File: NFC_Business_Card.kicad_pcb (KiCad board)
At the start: 2 copper layers, 85.6 x 54 mm, 7 parts

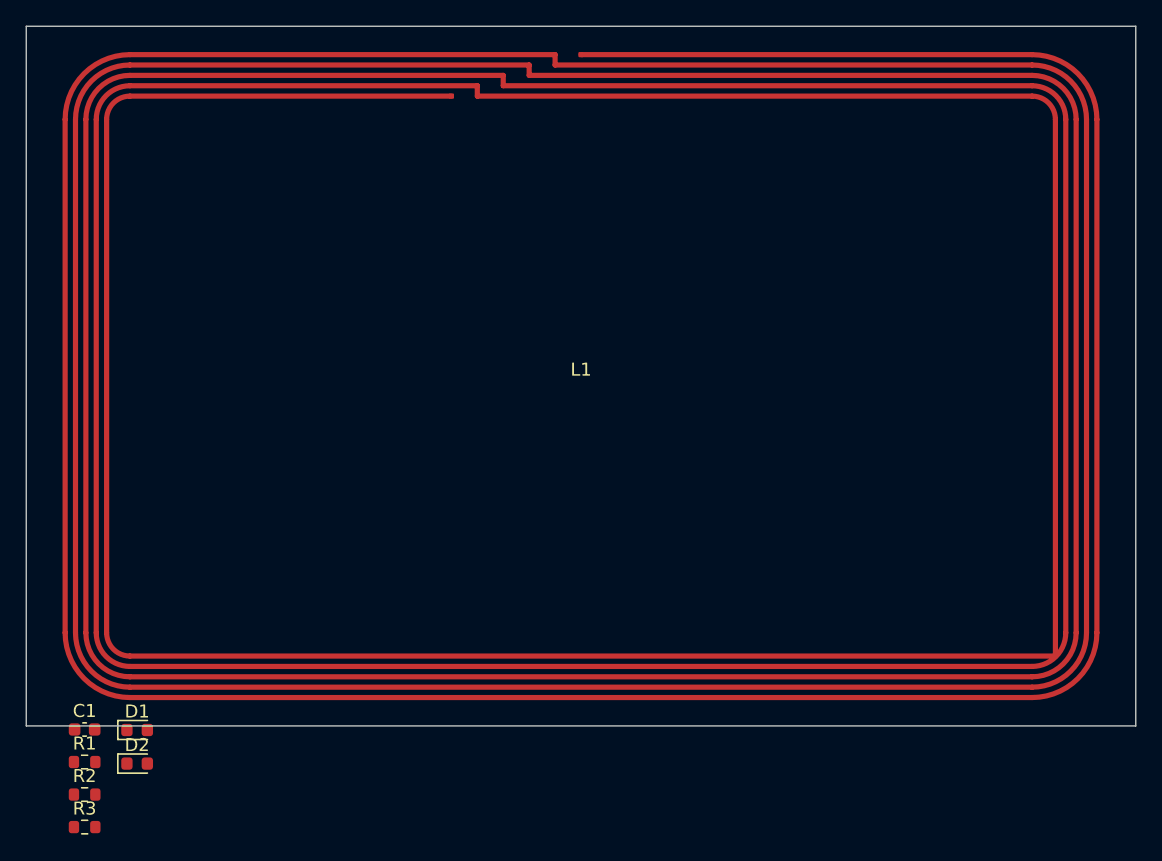
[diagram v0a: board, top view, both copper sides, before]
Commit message: Placed most components
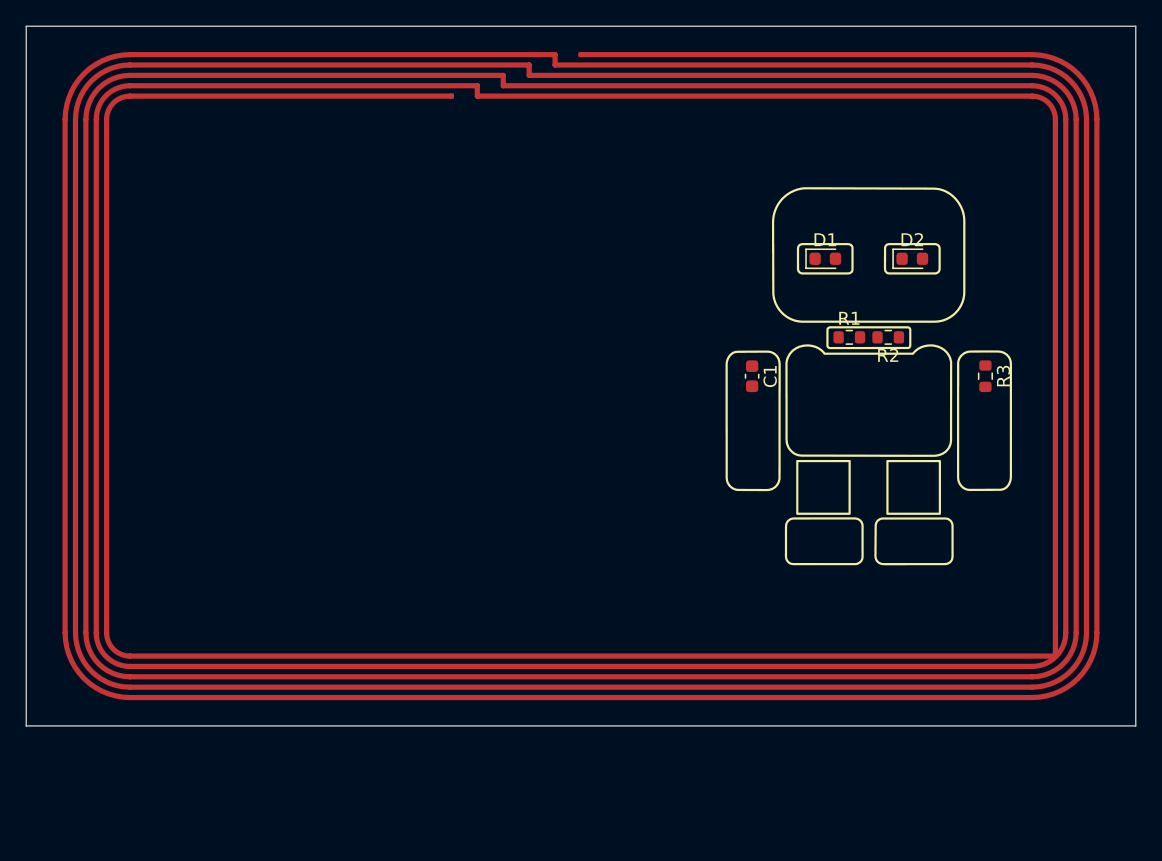
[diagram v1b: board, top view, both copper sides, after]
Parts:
- added G***: Ryan_Robot_Outline_29mm, NFC_Custom:Ryan_Robot_Outline_29mm, F.Cu at (115.0, 77.0)
- moved R3 77.7 mm to (124.0, 77.0), turned to -90 degrees
- moved D2 71.4 mm to (118.4, 67.9)
- moved R2 71.3 mm to (116.5, 74.0), turned to 180 degrees
- moved R1 67.5 mm to (113.5, 74.0)
- moved D1 64.3 mm to (111.6, 67.9)
- moved C1 58.3 mm to (106.0, 77.0), turned to -90 degrees
